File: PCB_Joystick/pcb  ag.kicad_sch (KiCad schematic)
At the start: 12 parts, among them J2 Conn_01x05, SW10 SW_Push_LED, SW6 SW_Push_LED, SW7 SW_Push_LED, SW8 SW_Push_LED, SW9 SW_Push_LED

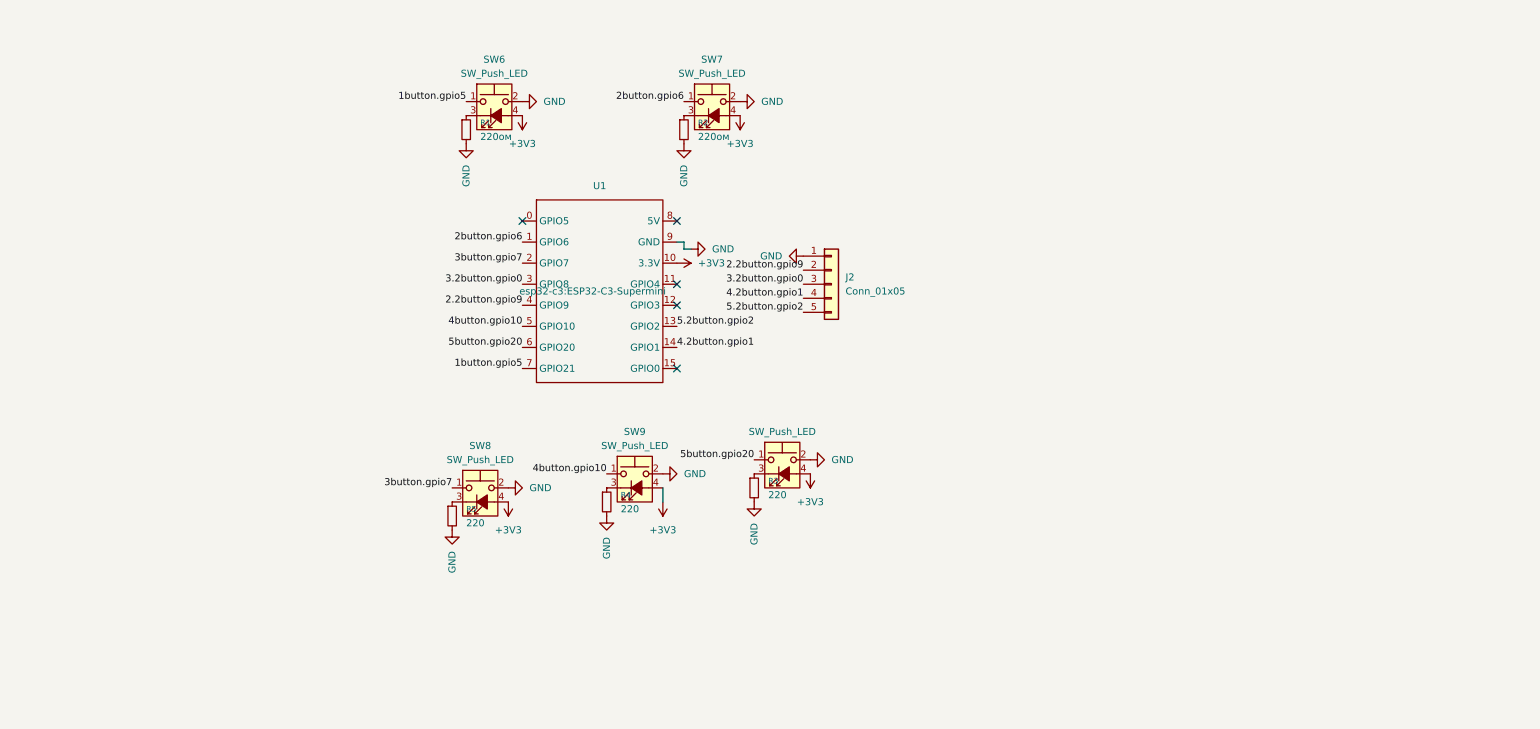
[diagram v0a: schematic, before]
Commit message: pcb
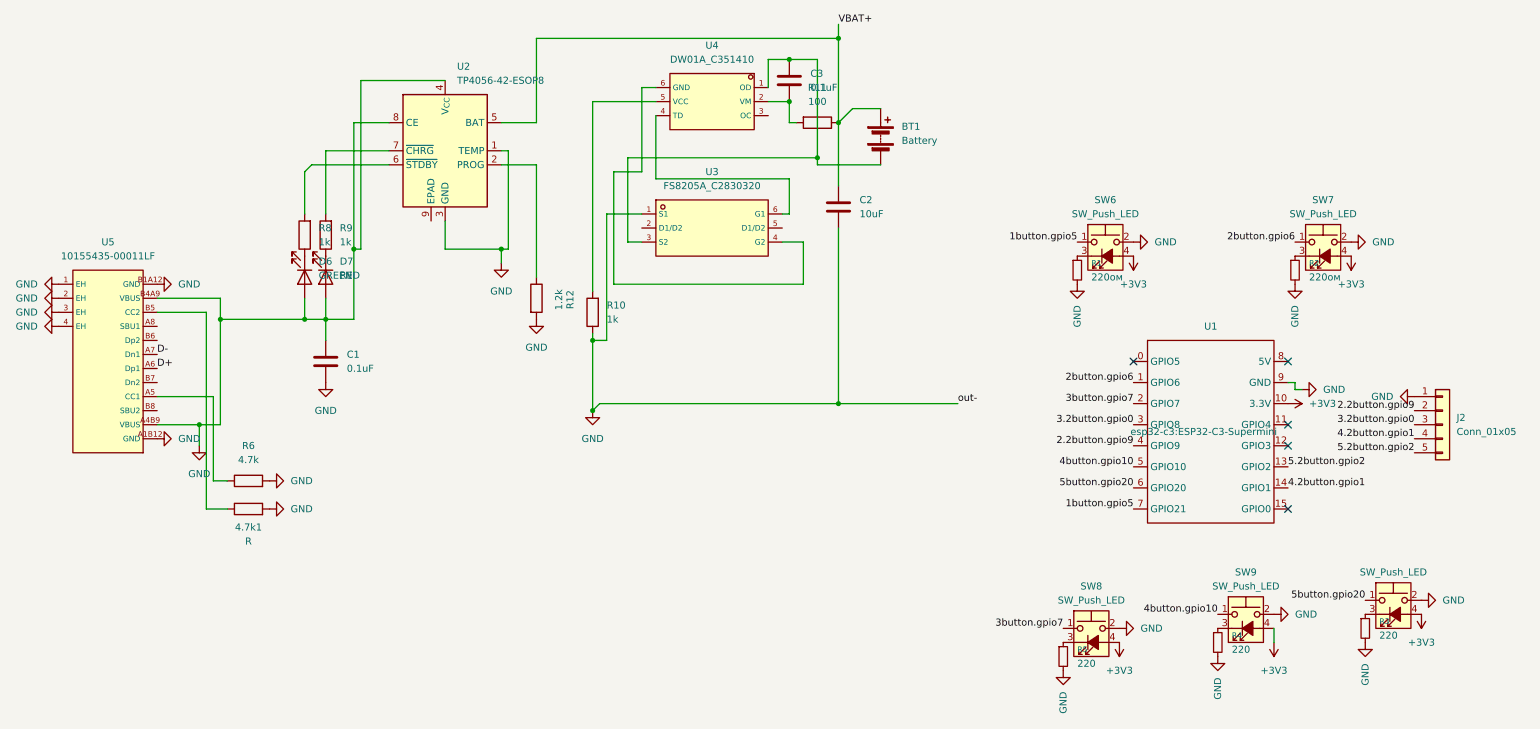
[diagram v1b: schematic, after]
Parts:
- added 4.7k1: R, Resistor_SMD:R_0603_1608Metric_Pad0.98x0.95mm_HandSolder, symbol Device:R
- added BT1: Battery, Connector_PinHeader_2.54mm:PinHeader_1x02_P2.54mm_Vertical, symbol Device:Battery
- added C1, C3: 0.1uF, Capacitor_SMD:C_0603_1608Metric_Pad1.08x0.95mm_HandSolder, symbol Device:C
- added C2: 10uF, Capacitor_SMD:C_0603_1608Metric_Pad1.08x0.95mm_HandSolder, symbol Device:C
- added D6: GREEN, LED_SMD:LED_Cree-XHP50_3V_HighDensity, symbol Device:LED
- added D7: RED, LED_SMD:LED_Cree-XHP50_3V_HighDensity, symbol Device:LED
- added R10, R8, R9: 1k, Resistor_SMD:R_0603_1608Metric_Pad0.98x0.95mm_HandSolder, symbol Device:R
- added R11: 100, Resistor_SMD:R_0603_1608Metric_Pad0.98x0.95mm_HandSolder, symbol Device:R
- added R12: 1.2k, Resistor_SMD:R_0603_1608Metric_Pad0.98x0.95mm_HandSolder, symbol Device:R
- added R6: 4.7k, Resistor_SMD:R_0603_1608Metric_Pad0.98x0.95mm_HandSolder, symbol Device:R
- added U2: TP4056-42-ESOP8, footprint:ESOP-8_L4.9-W3.9-P1.27-LS6.0-BL-EP, symbol Battery_Management:TP4056-42-ESOP8
- added U3: FS8205A_C2830320, footprint:SOT-23-6_L2.9-W1.6-P0.95-LS2.8-BR, symbol FS8205A_C2830320:FS8205A_C2830320
- added U4: DW01A_C351410, footprint:SOT-23-6_L2.9-W1.6-P0.95-LS2.8-BL, symbol DW01A_C351410:DW01A_C351410
- added U5: 10155435-00011LF, footprint:USB-C-SMD_10155435-00011LF, symbol 10155435-00011LF:10155435-00011LF
- R1, R2, R3, R4, R5: footprint Resistor_THT:R_Axial_DIN0207_L6.3mm_D2.5mm_P7.62mm_Horizontal -> Resistor_SMD:R_0603_1608Metric_Pad0.98x0.95mm_HandSolder
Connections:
- net GND: now also 4.7k1.2, C1.1, C1.2, C2.2, D6.2 (A), D7.2 (A), R10.1, R12.2, R6.2, U2.1 (TEMP), U2.3 (GND), U2.4 (V_{CC}), U2.8 (CE), U3.1 (S1), U5.1 (EH), U5.2 (EH), U5.3 (EH), U5.4 (EH), U5.A1B12 (GND), U5.A4B9 (VBUS), U5.B1A12 (GND), U5.B4A9 (VBUS)
- new net: D7.1 (K), R9.1
- new net: D6.1 (K), R8.1
- new net: R10.2, U4.5 (VCC)
- new net: R8.2, U2.6 (~{STDBY})
- new net: BT1.2 (-), C3.1, U3.3 (S2), U4.1 (OD)
- new net: C3.2, R11.2, U4.2 (VM)
- new net: U3.6 (G1), U4.4 (TD)
- new net: U3.4 (G2), U4.6 (GND)
- new net: R12.1, U2.2 (PROG)
- new net: R9.2, U2.7 (~{CHRG})
- new net: 4.7k1.1, U5.B5 (CC2)
- new net: R6.1, U5.A5 (CC1)
- new net D+: U5.A6 (Dp1)
- new net D-: U5.A7 (Dn1)
- new net VBAT+: BT1.1 (+), C2.1, R11.1, U2.5 (BAT)
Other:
- moved on the sheet: J2, R1, R2, R3, R4, R5, SW6, SW7, SW8, SW9, U1

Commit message: UPD
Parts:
- D6, D7: footprint LED_SMD:LED_Cree-XHP50_3V_HighDensity -> LED_SMD:LED_0603_1608Metric_Pad1.05x0.95mm_HandSolder
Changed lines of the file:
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@@
 			)
 		)
-		(property "Footprint" "LED_SMD:LED_Cree-XHP50_3V_HighDensity"
+		(property "Footprint" "LED_SMD:LED_0603_1608Metric_Pad1.05x0.95mm_HandSolder"
 			(at 73.66 81.28 0)
 			(hide yes)
@@
 			)
 		)
-		(property "Footprint" "LED_SMD:LED_Cree-XHP50_3V_HighDensity"
+		(property "Footprint" "LED_SMD:LED_0603_1608Metric_Pad1.05x0.95mm_HandSolder"
 			(at 69.85 81.28 0)
 			(hide yes)
